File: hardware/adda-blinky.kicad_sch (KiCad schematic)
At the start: 18 parts, among them J1 Conn_01x02, J2 Conn_01x02, J3 USB_B_Micro, J4 Conn_01x02, U1 ATtiny1616-S, U2 ATtiny1616-M, U3 AMS1117-3.3

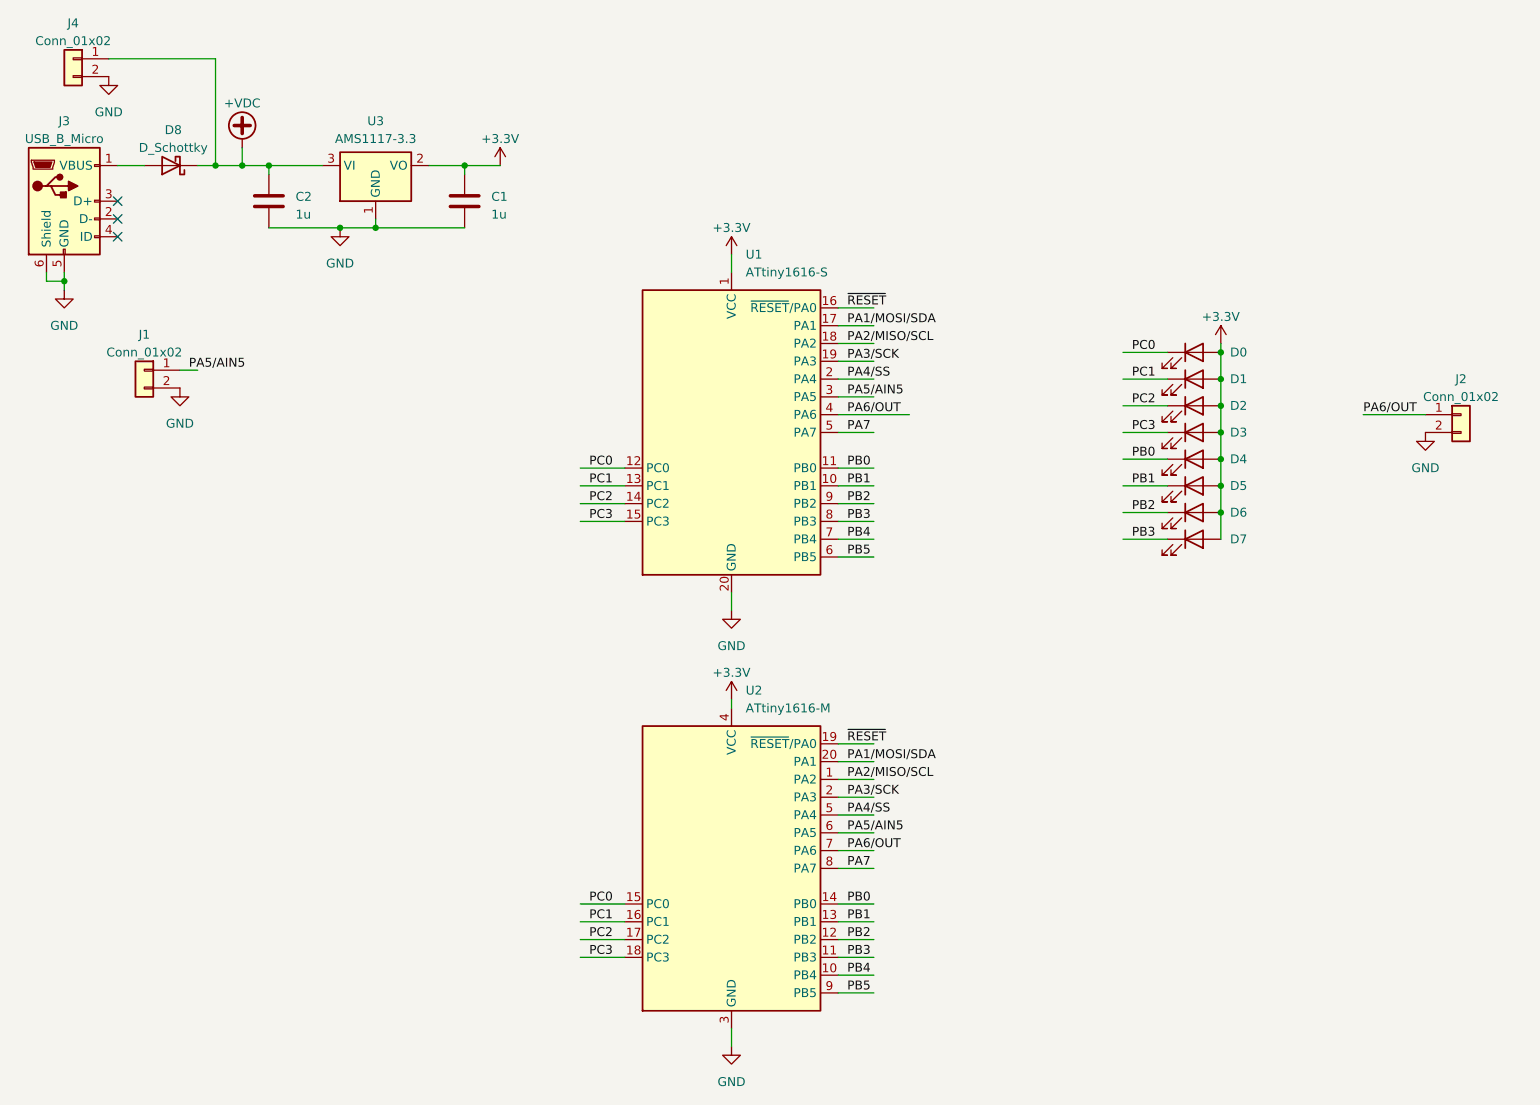
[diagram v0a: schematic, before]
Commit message: First order
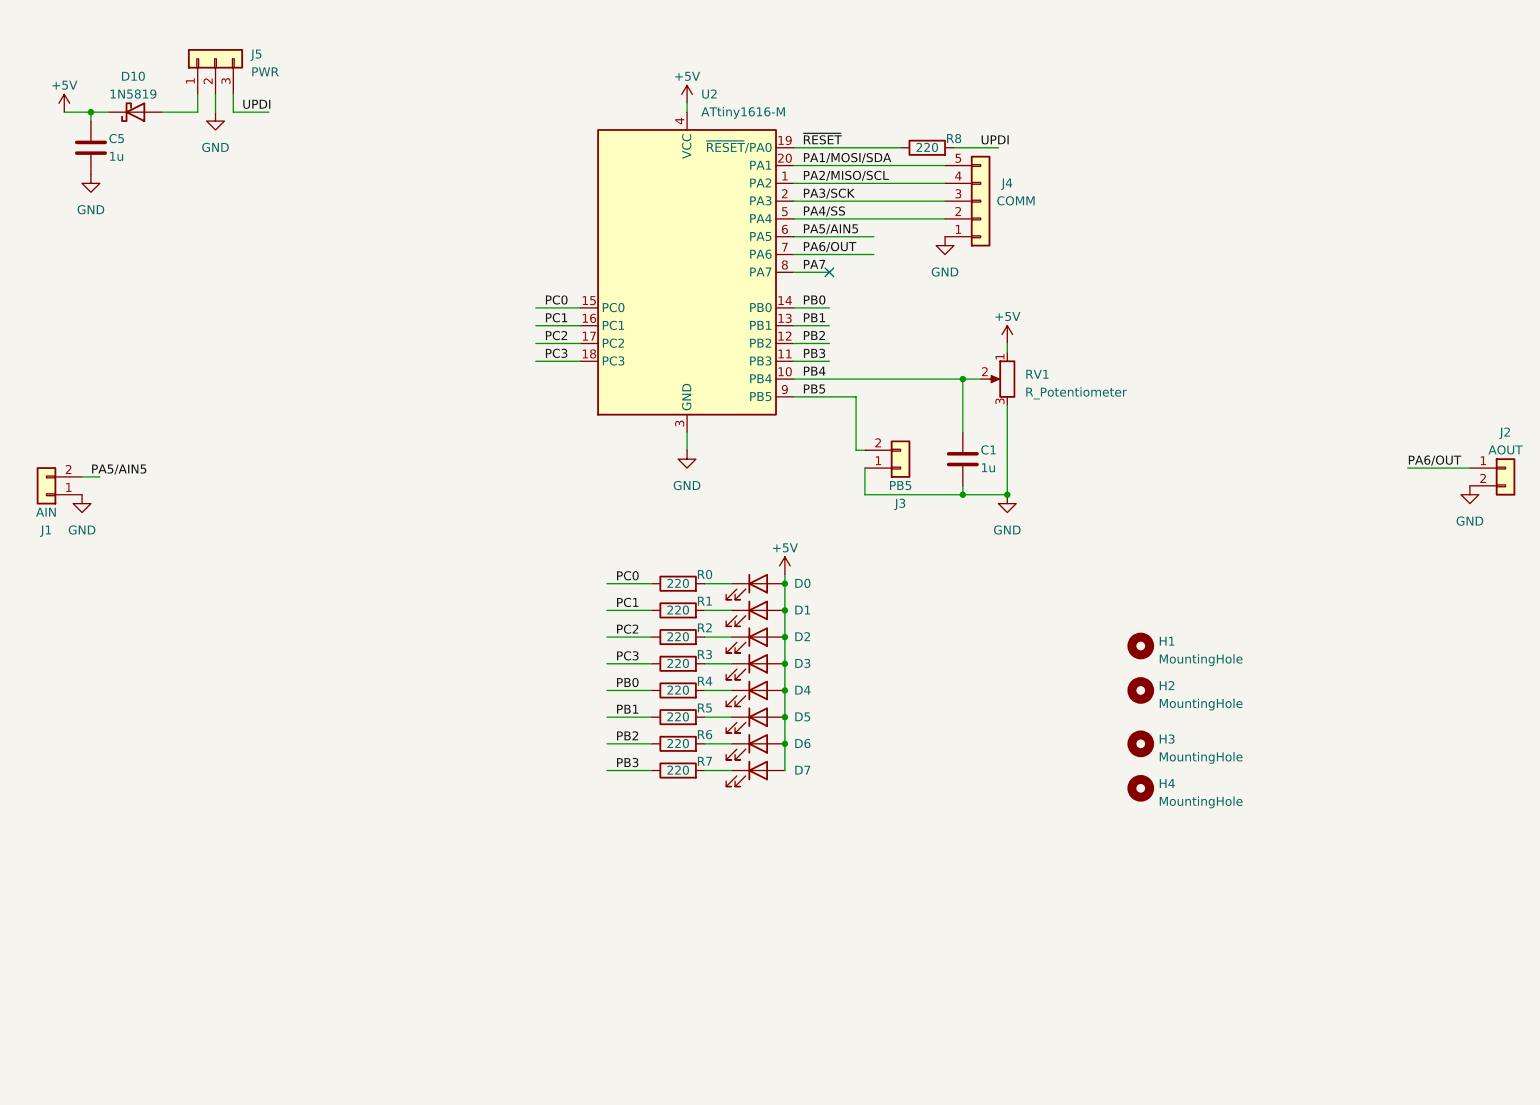
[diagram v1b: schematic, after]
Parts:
- removed C2: 1u, Capacitor_SMD:C_0805_2012Metric, symbol Device:C
- removed D8: D_Schottky, symbol Device:D_Schottky
- removed J3: USB_B_Micro, Connector_USB:USB_Micro-AB_Molex_47590-0001, symbol Connector:USB_B_Micro
- removed J4: Conn_01x02, Connector_Molex:Molex_KK-254_AE-6410-02A_1x02_P2.54mm_Vertical, symbol Connector_Generic:Conn_01x02
- removed U1: ATtiny1616-S, Package_SO:SOIC-20W_7.5x12.8mm_P1.27mm, symbol MCU_Microchip_ATtiny:ATtiny1616-S
- removed U3: AMS1117-3.3, Package_TO_SOT_SMD:SOT-223-3_TabPin2, symbol Regulator_Linear:AMS1117-3.3
- added C5: 1u, Capacitor_SMD:C_0805_2012Metric, symbol Device:C
- added D10: 1N5819, Diode_SMD:D_SOD-323, symbol Device:D_Schottky
- added H1: MountingHole, MountingHole:MountingHole_3.2mm_M3_Pad, symbol Mechanical:MountingHole
- added H2, H3, H4: MountingHole, symbol Mechanical:MountingHole
- added J3: PB5, Connector_Molex:Molex_KK-254_AE-6410-02A_1x02_P2.54mm_Vertical, symbol Connector_Generic:Conn_01x02
- added J4: COMM, Connector_Molex:Molex_KK-254_AE-6410-05A_1x05_P2.54mm_Vertical, symbol Connector_Generic:Conn_01x05
- added J5: PWR, Connector_Molex:Molex_KK-254_AE-6410-03A_1x03_P2.54mm_Vertical, symbol Connector_Generic:Conn_01x03
- added R0, R1, R2, R3, R4, R5, R6, R7, R8: 220, Resistor_SMD:R_0805_2012Metric, symbol Device:R
- added RV1: R_Potentiometer, Connector_PinHeader_2.54mm:PinHeader_1x03_P2.54mm_Vertical, symbol Device:R_Potentiometer
- J1: value Conn_01x02 -> AIN
- J2: value Conn_01x02 -> AOUT
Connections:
- net GND: now also J1.1 (Pin_1), C5.2, J3.1 (Pin_1), J4.1 (Pin_1), J5.2 (Pin_2), RV1.3; no longer J1.2 (Pin_2)
- net PA1/MOSI/SDA: now also J4.5 (Pin_5)
- net PA2/MISO/SCL: now also J4.4 (Pin_4)
- net PA3/SCK: now also J4.3 (Pin_3)
- net PA4/SS: now also J4.2 (Pin_2)
- net PA5/AIN5: now also J1.2 (Pin_2); no longer J1.1 (Pin_1)
- net PB0: now also R4.1; no longer D4.1 (K)
- net PB1: now also R5.1; no longer D5.1 (K)
- net PB2: now also R6.1; no longer D6.1 (K)
- net PB3: now also R7.1; no longer D7.1 (K)
- net PB4: now also C1.1, RV1.2
- net PB5: now also J3.2 (Pin_2)
- net PC0: now also R0.1; no longer D0.1 (K)
- net PC1: now also R1.1; no longer D1.1 (K)
- net PC2: now also R2.1; no longer D2.1 (K)
- net PC3: now also R3.1; no longer D3.1 (K)
- net ~{RESET}: now also R8.1
- net +3.3V renamed +5V
- net +5V: now also C5.1, D10.1 (K), RV1.1; no longer C1.1
- new net: D6.1 (K), R6.2
- new net: D7.1 (K), R7.2
- new net: D2.1 (K), R2.2
- new net: D10.2 (A), J5.1 (Pin_1)
- new net: D5.1 (K), R5.2
- new net: D3.1 (K), R3.2
- new net: D0.1 (K), R0.2
- new net: D4.1 (K), R4.2
- new net: D1.1 (K), R1.2
- new net UPDI: J5.3 (Pin_3), R8.2
- no-connect marks 3 -> 1
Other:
- moved on the sheet: D0, D1, D2, D3, D4, D5, D6, D7, J1, J2, U2
